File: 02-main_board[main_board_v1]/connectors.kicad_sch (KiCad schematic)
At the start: 3 parts, among them J1 2-84952-0, J2 2-84952-4, J3 FH41-15S-0.5SH_05_

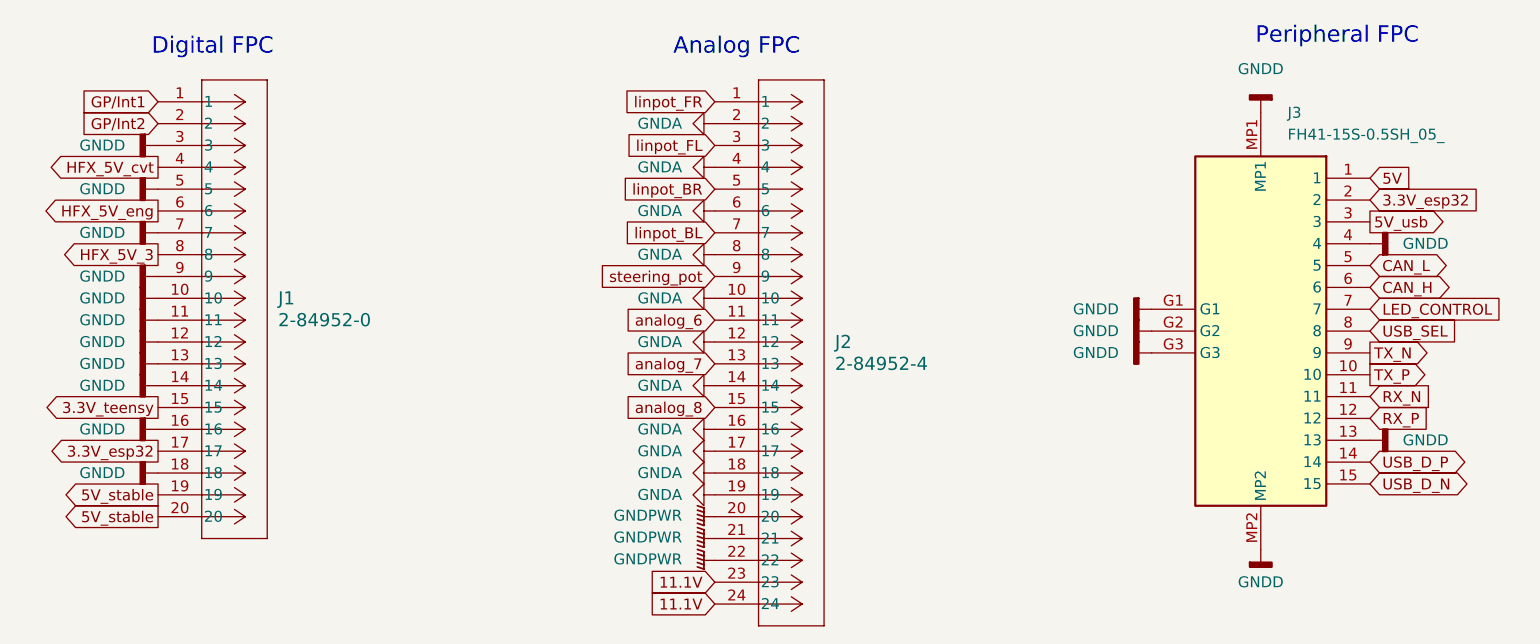
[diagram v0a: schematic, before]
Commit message: first rev
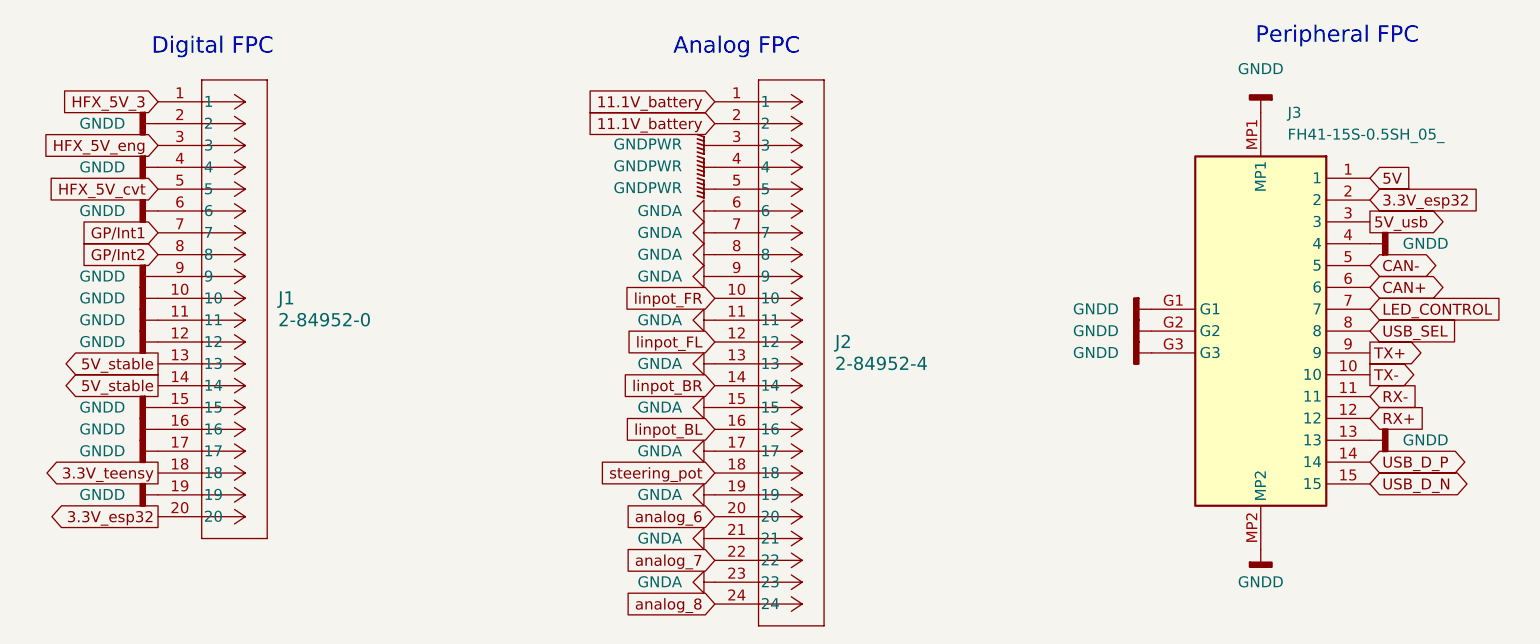
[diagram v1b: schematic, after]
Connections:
- net 3.3V_esp32: now also J1.20; no longer J1.17
- net 3.3V_teensy: now also J1.18; no longer J1.15
- net 5V_stable: now also J1.13, J1.14; no longer J1.19, J1.20
- net GNDA: now also J2.11, J2.13, J2.15, J2.21, J2.23, J2.7, J2.9; no longer J2.10, J2.12, J2.14, J2.16, J2.18, J2.2, J2.4
- net GNDD: now also J1.15, J1.17, J1.19, J1.2, J1.4, J1.6; no longer J1.13, J1.14, J1.18, J1.3, J1.5, J1.7
- net GNDPWR: now also J2.3, J2.4, J2.5; no longer J2.20, J2.21, J2.22
- net GP/Int1: now also J1.7; no longer J1.1
- net GP/Int2: now also J1.8; no longer J1.2
- net HFX_5V_3: now also J1.1; no longer J1.8
- net HFX_5V_cvt: now also J1.5; no longer J1.4
- net HFX_5V_eng: now also J1.3; no longer J1.6
- net analog_6: now also J2.20; no longer J2.11
- net analog_7: now also J2.22; no longer J2.13
- net analog_8: now also J2.24; no longer J2.15
- net linpot_BL: now also J2.16; no longer J2.7
- net linpot_BR: now also J2.14; no longer J2.5
- net linpot_FL: now also J2.12; no longer J2.3
- net linpot_FR: now also J2.10; no longer J2.1
- net steering_pot: now also J2.18; no longer J2.9
- removed net 11.1V: J2.23, J2.24
- net CAN_H renamed CAN+
- net CAN_L renamed CAN-
- net RX_N renamed RX-
- net RX_P renamed RX+
- net TX_N renamed TX+
- net TX_P renamed TX-
- new net 11.1V_battery: J2.1, J2.2
